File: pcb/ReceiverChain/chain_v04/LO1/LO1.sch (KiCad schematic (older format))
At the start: 65 parts, among them J1 RF-IN, J2 LO1, J3 GND, J4 VDD, J5 IF TEST, J6 LO2, J7 RF-OUT, U1 LP3985IM5-5.0, U10 NFL21SP106X1C3D, U2 SKY67159, U3 LT5526, U4 TPS79933, U5 PAT0816, U6 MEM2012V121R, U7 B39921, U8 PAT0816, U9 LT5526

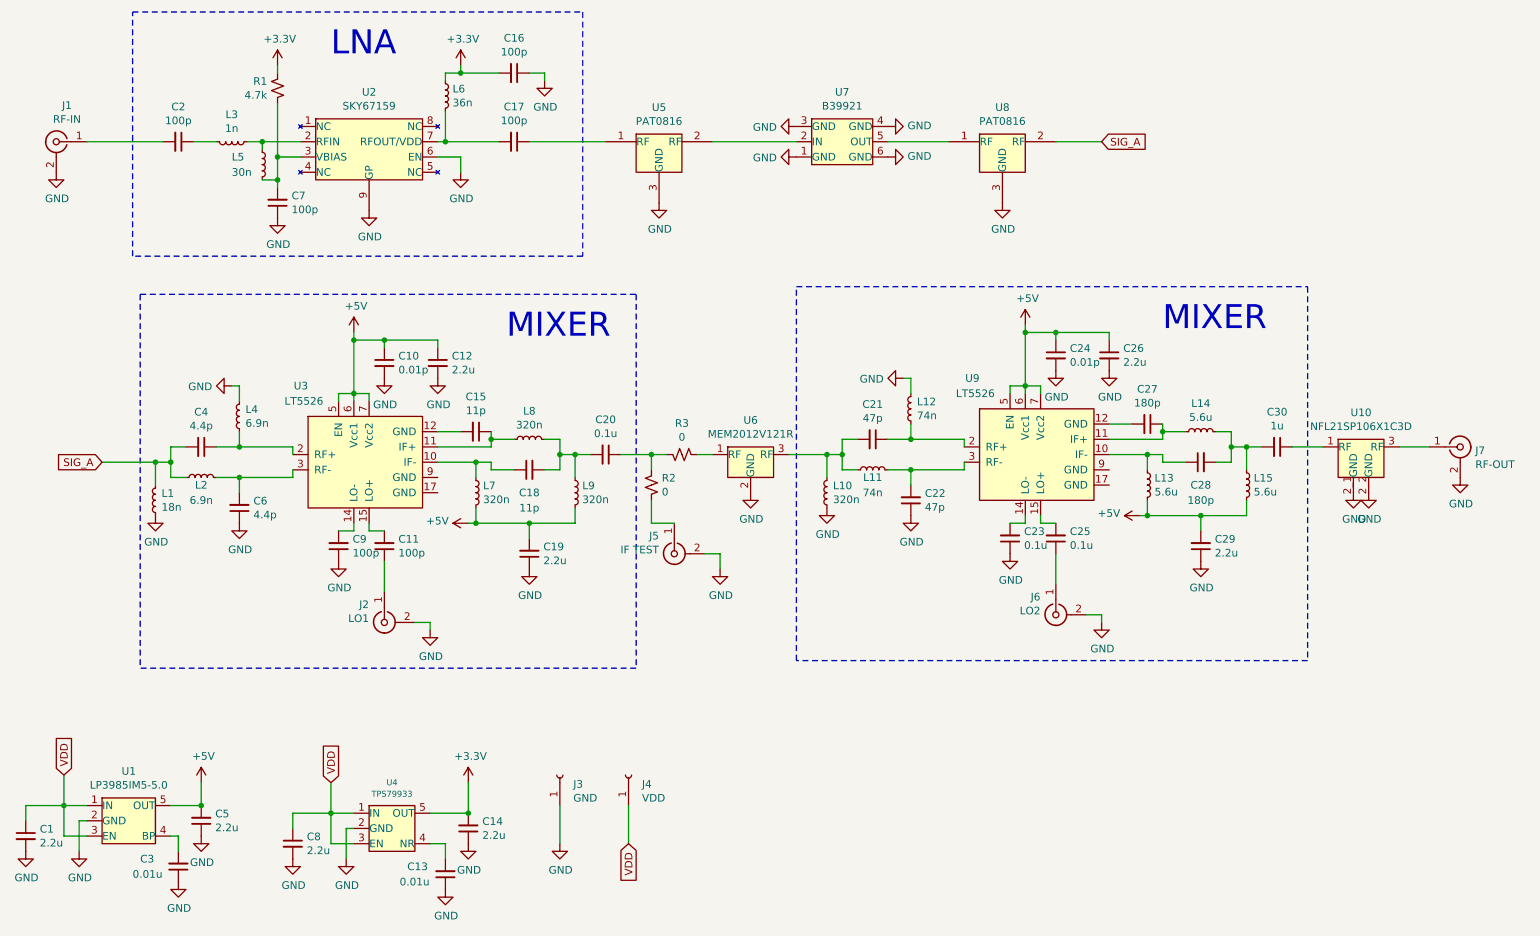
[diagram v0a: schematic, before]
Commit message: yea
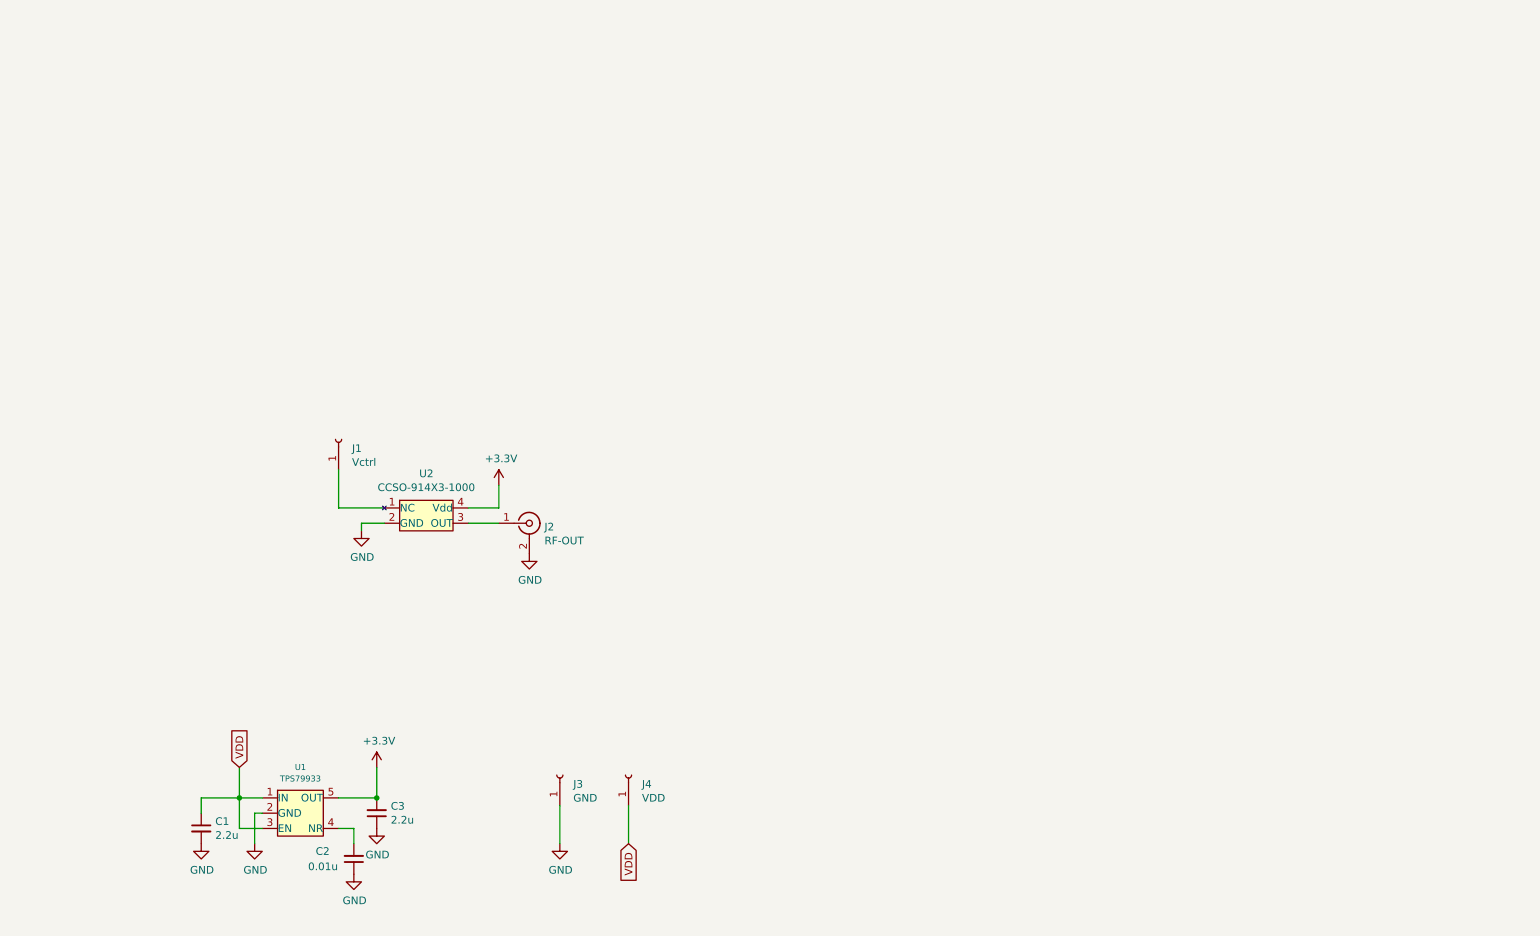
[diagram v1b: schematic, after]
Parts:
- removed C1: 2.2u, Connector_Wire:SolderWirePad_1x01_Drill0.8mm, symbol Device:C_Small
- removed C10, C24: 0.01p, symbol Device:C_Small
- removed C11, C16, C17, C2, C7, C9: 100p, symbol Device:C_Small
- removed C12, C19, C26, C29, C5: 2.2u, symbol Device:C_Small
- removed C15, C18: 11p, symbol Device:C_Small
- removed C20, C23, C25: 0.1u, symbol Device:C_Small
- removed C21, C22: 47p, symbol Device:C_Small
- removed C27, C28: 180p, symbol Device:C_Small
- removed C3: 0.01u, symbol Device:C_Small
- removed C30: 1u, symbol Device:C_Small
- removed C4, C6: 4.4p, symbol Device:C_Small
- removed J1: RF-IN, symbol Connector:Conn_Coaxial
- removed J2: LO1, symbol Connector:Conn_Coaxial
- removed J5: IF TEST, symbol Connector:Conn_Coaxial
- removed J6: LO2, symbol Connector:Conn_Coaxial
- removed L1: 18n, symbol Device:L_Small
- removed L10, L7, L8, L9: 320n, symbol Device:L_Small
- removed L11, L12: 74n, symbol Device:L_Small
- removed L13, L14, L15: 5.6u, symbol Device:L_Small
- removed L2, L4: 6.9n, symbol Device:L_Small
- removed L3: 1n, symbol Device:L_Small
- removed L5: 30n, symbol Device:L_Small
- removed L6: 36n, symbol Device:L_Small
- removed R1: 4.7k, symbol Device:R_Small_US
- removed R2, R3: 0, symbol Device:R_Small_US
- removed U1: LP3985IM5-5.0, symbol chain:LP3985IM5-5.0
- removed U10: NFL21SP106X1C3D, symbol chain:NFL21SP106X1C3D
- removed U2: SKY67159, symbol chain:SKY67159-396LF
- removed U3, U9: LT5526, symbol chain:LT5526
- removed U5, U8: PAT0816, symbol chain:PAT0816
- removed U6: MEM2012V121R, symbol chain:MEM2012V121R
- removed U7: B39921, symbol chain:B39921
- added J1: Vctrl, Connector_Wire:SolderWirePad_1x01_Drill0.8mm, symbol Connector:Conn_01x01_Female
- added U2: CCSO-914X3-1000, OSCSC508P1420X914X530-4N:OSCSC508P1420X914X530-4N, symbol chain:CCSO-914X3-1000
- C1: renamed from C8; footprint (none) -> Capacitor_SMD:C_0805_2012Metric
- C2: renamed from C13; footprint (none) -> Capacitor_SMD:C_0805_2012Metric
- C3: renamed from C14; footprint (none) -> Capacitor_SMD:C_0805_2012Metric
- J2: renamed from J7; footprint (none) -> footprints:sma-edge-small
- U1: renamed from U4; footprint (none) -> LP3985IM5-5.0:SOT95P300X120-5N
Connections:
- net +3V3: now also U2.4 (Vdd)
- net GND: now also U2.2 (GND)
- net at J2.1 (In): now also U2.3 (OUT)
- new net: J1.1 (Pin_1), U2.1 (NC)
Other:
- note removed: "LNA"
- note removed: "MIXER"
- moved on the sheet: C1, C2, C3, J2, U1
